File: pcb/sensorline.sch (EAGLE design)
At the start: 19 parts, among them X1 FH12-14S-0.5SH

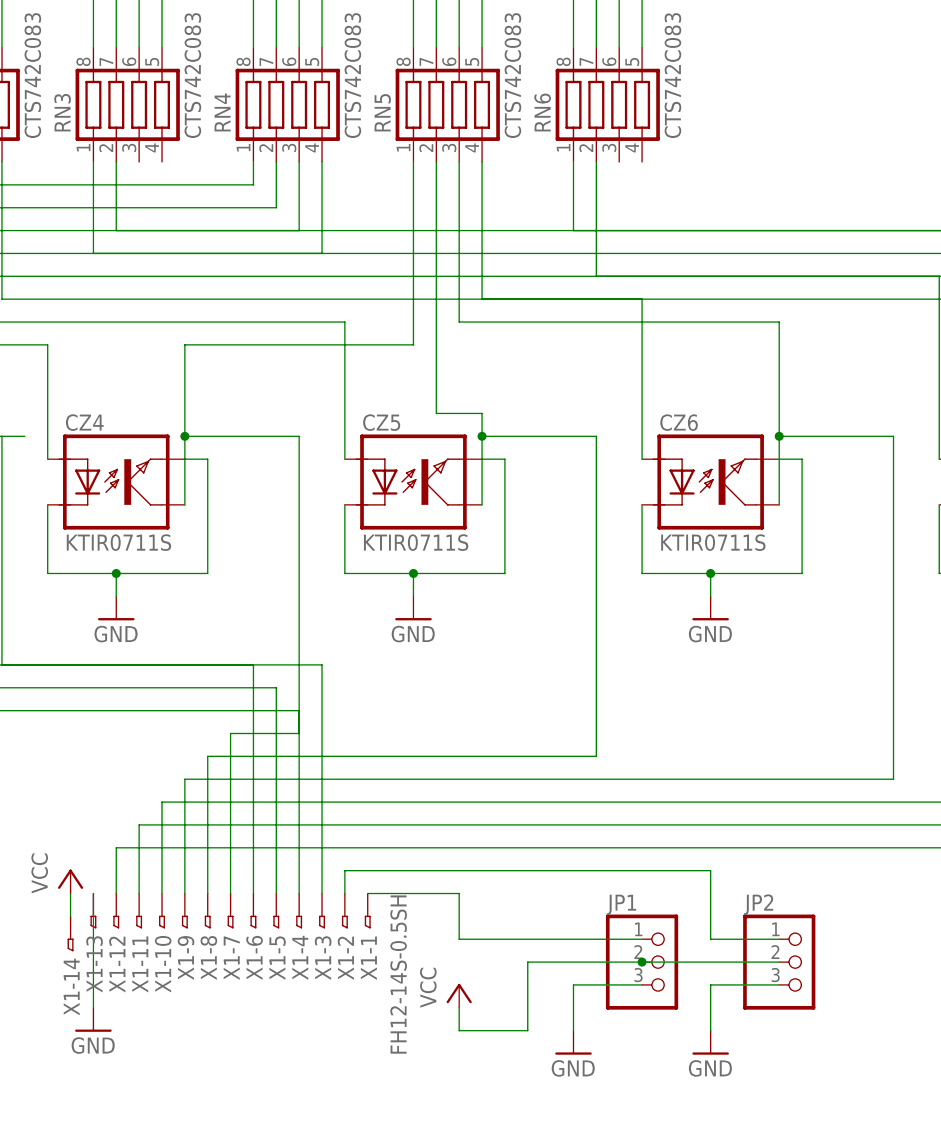
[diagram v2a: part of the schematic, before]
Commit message: hard level
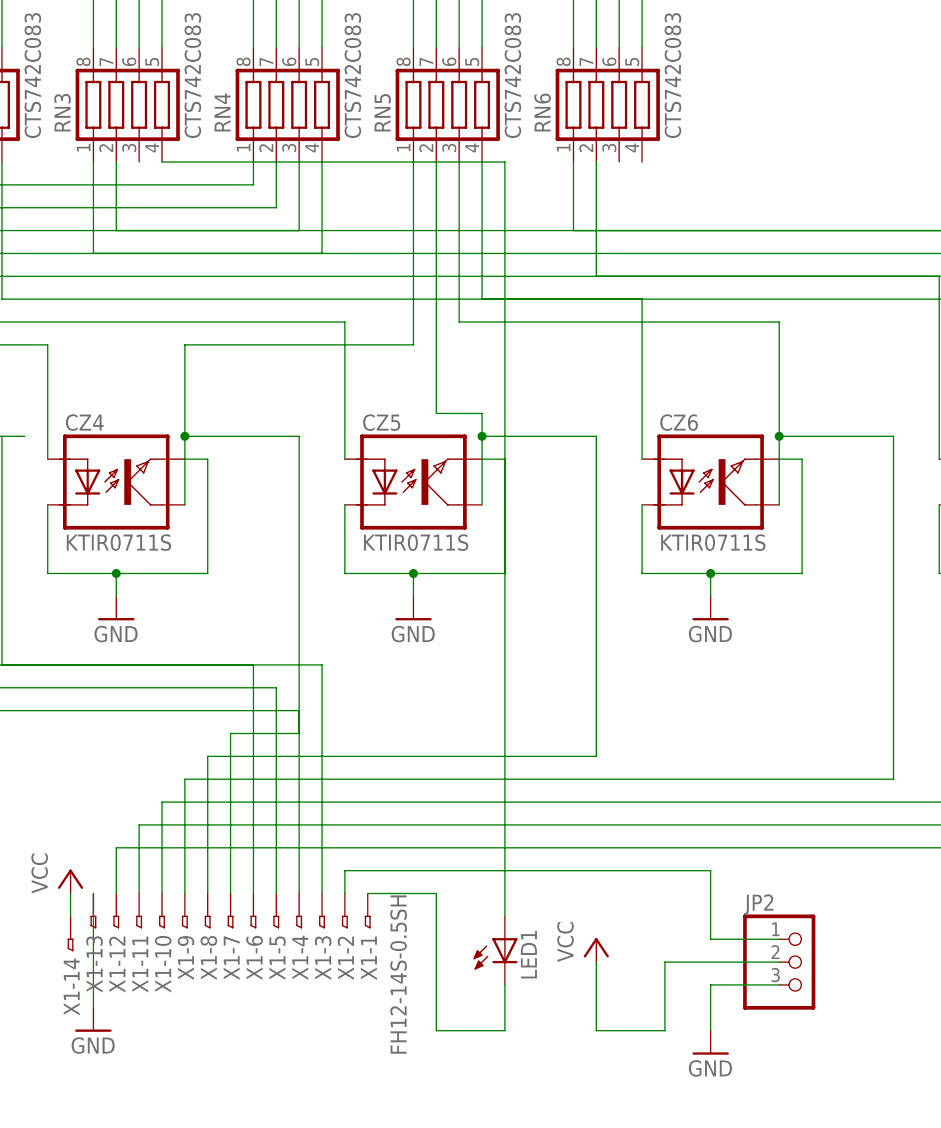
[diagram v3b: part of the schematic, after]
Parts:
- removed JP1: (no value), pinhead:PINHD-1X3
- added LED1: (no value), led:LEDCHIPLED_0603
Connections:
- new net N$23: LED1.C, X1-1.1
- net GND: no longer JP1.3
- net N$21: now also LED1.A, RN3.4; no longer JP1.1, X1-1.1
- net VCC: no longer JP1.2
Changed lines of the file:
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@@
 <?xml version="1.0" encoding="utf-8"?>
 <!DOCTYPE eagle SYSTEM "eagle.dtd">
-<eagle version="8.1.1">
+<eagle version="8.1.0">
 <drawing>
 <settings>
@@
 <part name="FRAME1" library="frames" deviceset="DINA3_L" device=""/>
 <part name="X1" library="con-hirose" deviceset="FH12-14S-0.5S" device="H"/>
-<part name="JP1" library="pinhead" deviceset="PINHD-1X3" device=""/>
 <part name="JP2" library="pinhead" deviceset="PINHD-1X3" device=""/>
 <part name="P+12" library="supply1" deviceset="VCC" device=""/>
-<part name="GND12" library="supply1" deviceset="GND" device=""/>
 <part name="GND13" library="supply1" deviceset="GND" device=""/>
 <part name="RN1" library="resistor-net" deviceset="CTS742C083" device=""/>
@@
 <part name="RN6" library="resistor-net" deviceset="CTS742C083" device=""/>
 <part name="P+1" library="supply1" deviceset="VCC" device=""/>
+<part name="LED1" library="led" deviceset="LED" device="CHIPLED_0603"/>
 </parts>
 <sheets>
@@
 <instance part="X1" gate="-13" x="83.82" y="45.72" rot="R270"/>
 <instance part="X1" gate="-14" x="81.28" y="43.18" rot="R270"/>
-<instance part="JP1" gate="A" x="147.32" y="40.64"/>
 <instance part="JP2" gate="A" x="162.56" y="40.64"/>
-<instance part="P+12" gate="VCC" x="124.46" y="38.1"/>
-<instance part="GND12" gate="1" x="137.16" y="30.48"/>
+<instance part="P+12" gate="VCC" x="139.7" y="43.18"/>
 <instance part="GND13" gate="1" x="152.4" y="30.48"/>
 <instance part="RN1" gate="G$1" x="50.8" y="134.62" rot="R90"/>
@@
 <instance part="RN6" gate="G$1" x="139.7" y="134.62" rot="R90"/>
 <instance part="P+1" gate="VCC" x="96.52" y="160.02"/>
+<instance part="LED1" gate="G$1" x="129.54" y="43.18"/>
 </instances>
 <busses>
@@
 </segment>
 <segment>
-<pinref part="JP1" gate="A" pin="3"/>
-<wire x1="144.78" y1="38.1" x2="137.16" y2="38.1" width="0.1524" layer="91"/>
-<wire x1="137.16" y1="38.1" x2="137.16" y2="33.02" width="0.1524" layer="91"/>
-<pinref part="GND12" gate="1" pin="GND"/>
-</segment>
-<segment>
 <pinref part="JP2" gate="A" pin="3"/>
 <wire x1="160.02" y1="38.1" x2="152.4" y2="38.1" width="0.1524" layer="91"/>
@@
 <segment>
 <pinref part="JP2" gate="A" pin="2"/>
-<pinref part="JP1" gate="A" pin="2"/>
-<wire x1="160.02" y1="40.64" x2="144.78" y2="40.64" width="0.1524" layer="91"/>
-<wire x1="144.78" y1="40.64" x2="132.08" y2="40.64" width="0.1524" layer="91"/>
-<wire x1="132.08" y1="40.64" x2="132.08" y2="33.02" width="0.1524" layer="91"/>
-<junction x="144.78" y="40.64"/>
-<wire x1="132.08" y1="33.02" x2="124.46" y2="33.02" width="0.1524" layer="91"/>
-<wire x1="124.46" y1="33.02" x2="124.46" y2="35.56" width="0.1524" layer="91"/>
+<wire x1="160.02" y1="40.64" x2="147.32" y2="40.64" width="0.1524" layer="91"/>
+<wire x1="147.32" y1="40.64" x2="147.32" y2="33.02" width="0.1524" layer="91"/>
+<wire x1="147.32" y1="33.02" x2="139.7" y2="33.02" width="0.1524" layer="91"/>
+<wire x1="139.7" y1="33.02" x2="139.7" y2="40.64" width="0.1524" layer="91"/>
 <pinref part="P+12" gate="VCC" pin="VCC"/>
 </segment>
@@
 </segment>
 </net>
-<net name="N$21" class="0">
-<segment>
-<pinref part="JP1" gate="A" pin="1"/>
-<wire x1="144.78" y1="43.18" x2="124.46" y2="43.18" width="0.1524" layer="91"/>
-<wire x1="124.46" y1="43.18" x2="124.46" y2="48.26" width="0.1524" layer="91"/>
-<pinref part="X1" gate="-1" pin="1"/>
-<wire x1="124.46" y1="48.26" x2="114.3" y2="48.26" width="0.1524" layer="91"/>
-</segment>
-</net>
 <net name="N$22" class="0">
 <segment>
@@
 </segment>
 </net>
+<net name="N$21" class="0">
+<segment>
+<pinref part="RN3" gate="G$1" pin="4"/>
+<wire x1="91.44" y1="129.54" x2="129.54" y2="129.54" width="0.1524" layer="91"/>
+<wire x1="129.54" y1="129.54" x2="129.54" y2="45.72" width="0.1524" layer="91"/>
+<pinref part="LED1" gate="G$1" pin="A"/>
+</segment>
+</net>
+<net name="N$23" class="0">
+<segment>
+<pinref part="LED1" gate="G$1" pin="C"/>
+<wire x1="129.54" y1="38.1" x2="129.54" y2="33.02" width="0.1524" layer="91"/>
+<wire x1="129.54" y1="33.02" x2="121.92" y2="33.02" width="0.1524" layer="91"/>
+<wire x1="121.92" y1="33.02" x2="121.92" y2="48.26" width="0.1524" layer="91"/>
+<pinref part="X1" gate="-1" pin="1"/>
+<wire x1="121.92" y1="48.26" x2="114.3" y2="48.26" width="0.1524" layer="91"/>
+</segment>
+</net>
